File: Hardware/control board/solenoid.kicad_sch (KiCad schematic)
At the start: 7 parts, among them J11 Screw_Terminal_01x02, Q3 NMOS

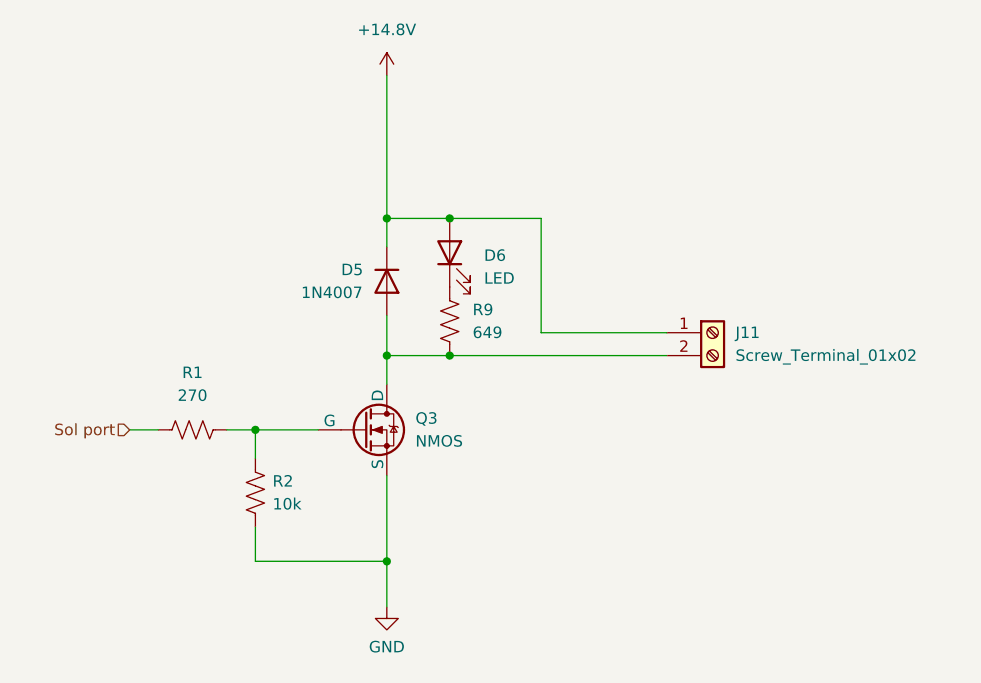
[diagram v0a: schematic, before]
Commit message: schematic formatted
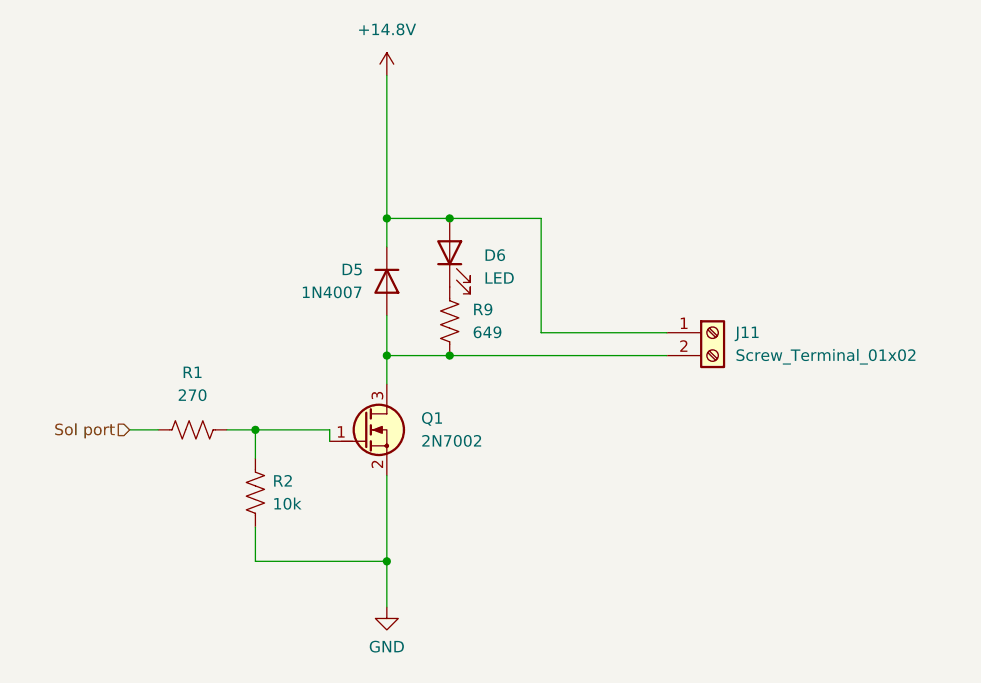
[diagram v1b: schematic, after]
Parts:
- removed Q3: NMOS, symbol Simulation_SPICE:NMOS
- added Q1: 2N7002, Package_TO_SOT_SMD_AKL:SOT-23, symbol PCM_Transistor_MOSFET_AKL:2N7002
- D6: footprint (none) -> LED_THT:LED_D3.0mm
- J11: footprint (none) -> TerminalBlock_Phoenix:TerminalBlock_Phoenix_MPT-0,5-2-2.54_1x02_P2.54mm_Horizontal
- R1, R2, R9: footprint (none) -> Resistor_SMD:R_0805_2012Metric
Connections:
- net GND: now also Q1.2 (S)
- net at D5.2 (A), J11.2 (Pin_2), R9.2: now also Q1.3 (D)
- net at R1.2, R2.1: now also Q1.1 (G)
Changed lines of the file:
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@@
     (stroke (width 0) (type default))
   )
-  (wire (pts (xy 107.95 99.06) (xy 114.935 99.06))
+  (wire (pts (xy 107.95 99.06) (xy 116.205 99.06))
     (stroke (width 0) (type default))
   )
@@
   )
   (wire (pts (xy 122.555 86.36) (xy 122.555 90.805))
+    (stroke (width 0) (type default))
+  )
+  (wire (pts (xy 116.205 99.06) (xy 116.205 100.33))
     (stroke (width 0) (type default))
   )
@@
     (effects (font (size 1.27 1.27)) (justify right))
   )
-  (symbol (lib_id "Simulation_SPICE:NMOS") (at 120.015 99.06 0) (unit 1)
-    (in_bom yes) (on_board yes) (dnp no) (fields_autoplaced)
-    (property "Reference" "Q3" (at 125.73 97.79 0)
-      (effects (font (size 1.27 1.27)) (justify left))
-    )
-    (property "Value" "NMOS" (at 125.73 100.33 0)
-      (effects (font (size 1.27 1.27)) (justify left))
-    )
-    (property "Footprint" "" (at 125.095 96.52 0)
-      (effects (font (size 1.27 1.27)) hide)
-    )
-    (property "Datasheet" "https://ngspice.sourceforge.io/docs/ngspice-manual.pdf" (at 120.015 111.76 0)
-      (effects (font (size 1.27 1.27)) hide)
-    )
-    (property "Sim.Device" "NMOS" (at 120.015 116.205 0)
-      (effects (font (size 1.27 1.27)) hide)
-    )
-    (property "Sim.Type" "VDMOS" (at 120.015 118.11 0)
-      (effects (font (size 1.27 1.27)) hide)
-    )
-    (property "Sim.Pins" "1=D 2=G 3=S" (at 120.015 114.3 0)
-      (effects (font (size 1.27 1.27)) hide)
-    )
-    (pin "1")
-    (pin "2")
-    (pin "3")
-    (instances
-      (project "solenoid"
-        (path "/b4ed5960-473e-41d7-9d87-eb439ed22219"
-          (reference "Q3") (unit 1)
-        )
-      )
-      (project "control board"
-        (path "/cf0863a8-7f64-449b-8eb4-3c06c871fb37"
-          (reference "Q3") (unit 1)
-        )
-        (path "/cf0863a8-7f64-449b-8eb4-3c06c871fb37/9fd0b45f-6f46-40af-ae0d-29c33b45e498"
-          (reference "Q1") (unit 1)
-        )
-        (path "/cf0863a8-7f64-449b-8eb4-3c06c871fb37/6163a064-c95f-47b6-9c17-0e18c391c233"
-          (reference "Q2") (unit 1)
-        )
-        (path "/cf0863a8-7f64-449b-8eb4-3c06c871fb37/f39ce93b-3626-4dde-a021-b00a2c8134c7"
-          (reference "Q3") (unit 1)
-        )
-      )
-    )
-  )
   (symbol (lib_id "Device:LED") (at 129.54 79.375 90) (unit 1)
     (in_bom yes) (on_board yes) (dnp no) (fields_autoplaced)
@@
       (effects (font (size 1.27 1.27)) (justify right))
     )
-    (property "Footprint" "" (at 129.54 79.375 0)
+    (property "Footprint" "LED_THT:LED_D3.0mm" (at 129.54 79.375 0)
       (effects (font (size 1.27 1.27)) hide)
     )
@@
         )
         (path "/cf0863a8-7f64-449b-8eb4-3c06c871fb37/9fd0b45f-6f46-40af-ae0d-29c33b45e498"
-          (reference "Green") (unit 1)
+          (reference "Green1") (unit 1)
         )
         (path "/cf0863a8-7f64-449b-8eb4-3c06c871fb37/6163a064-c95f-47b6-9c17-0e18c391c233"
@@
       (effects (font (size 1.27 1.27)) (justify left))
     )
-    (property "Footprint" "" (at 158.75 88.265 0)
+    (property "Footprint" "TerminalBlock_Phoenix:TerminalBlock_Phoenix_MPT-0,5-2-2.54_1x02_P2.54mm_Horizontal" (at 158.75 88.265 0)
       (effects (font (size 1.27 1.27)) hide)
     )
@@
       (effects (font (size 1.27 1.27)))
     )
-    (property "Footprint" "" (at 101.219 98.044 90)
+    (property "Footprint" "Resistor_SMD:R_0805_2012Metric" (at 101.219 98.044 90)
       (effects (font (size 1.27 1.27)) hide)
     )
@@
       (effects (font (size 1.27 1.27)) (justify left))
     )
-    (property "Footprint" "" (at 108.966 106.299 90)
+    (property "Footprint" "Resistor_SMD:R_0805_2012Metric" (at 108.966 106.299 90)
       (effects (font (size 1.27 1.27)) hide)
     )
@@
       (effects (font (size 1.27 1.27)) (justify left))
     )
-    (property "Footprint" "" (at 130.556 87.249 90)
+    (property "Footprint" "Resistor_SMD:R_0805_2012Metric" (at 130.556 87.249 90)
       (effects (font (size 1.27 1.27)) hide)
     )
@@
         )
       )
+    )
+  )
+  (symbol (lib_id "PCM_Transistor_MOSFET_AKL:2N7002") (at 120.015 99.06 0) (unit 1)
+    (in_bom yes) (on_board yes) (dnp no) (fields_autoplaced)
+    (property "Reference" "Q1" (at 126.365 97.79 0)
+      (effects (font (size 1.27 1.27)) (justify left))
+    )
+    (property "Value" "2N7002" (at 126.365 100.33 0)
+      (effects (font (size 1.27 1.27)) (justify left))
+    )
+    (property "Footprint" "Package_TO_SOT_SMD_AKL:SOT-23" (at 125.095 96.52 0)
+      (effects (font (size 1.27 1.27)) hide)
+    )
+    (property "Datasheet" "https://www.tme.eu/Document/7df5cae36abdfcedddb681f5be886f05/2N7000.pdf" (at 120.015 99.06 0)
+      (effects (font (size 1.27 1.27)) hide)
+    )
+    (pin "1")
+    (pin "2")
+    (pin "3")
+    (instances
+      (project "control board"
+        (path "/cf0863a8-7f64-449b-8eb4-3c06c871fb37/9fd0b45f-6f46-40af-ae0d-29c33b45e498"
+          (reference "Q1") (unit 1)
+        )
+        (path "/cf0863a8-7f64-449b-8eb4-3c06c871fb37/6163a064-c95f-47b6-9c17-0e18c391c233"
+          (reference "Q2") (unit 1)
+        )
+        (path "/cf0863a8-7f64-449b-8eb4-3c06c871fb37/f39ce93b-3626-4dde-a021-b00a2c8134c7"
+          (reference "Q3") (unit 1)
+        )
+      )

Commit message: Revert "Merge branch 'hardware' of https://github.com/bruin-underwater-robotics/2023-2024 into hardware"
This reverts commit f5050c74fbd2d727488e15b71bfb24c9149407df, reversing
changes made to d4ffa11f2369dfdbeb25d57bd1642de1ab50c466.
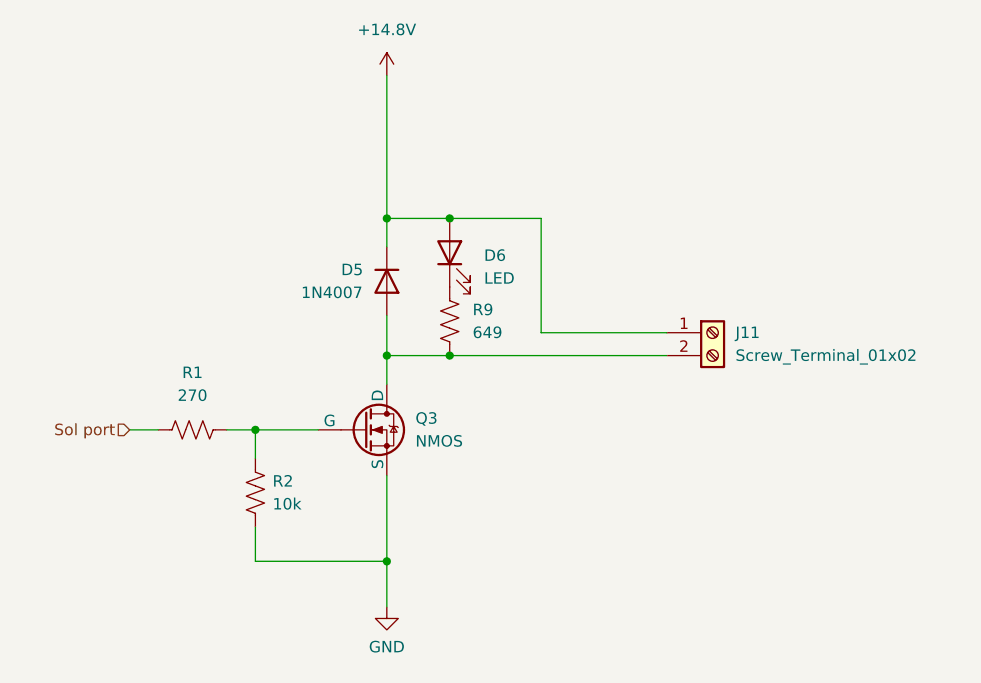
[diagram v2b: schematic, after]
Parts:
- removed Q1: 2N7002, Package_TO_SOT_SMD_AKL:SOT-23, symbol PCM_Transistor_MOSFET_AKL:2N7002
- added Q3: NMOS, symbol Simulation_SPICE:NMOS
- D6: footprint LED_THT:LED_D3.0mm -> (none)
- J11: footprint TerminalBlock_Phoenix:TerminalBlock_Phoenix_MPT-0,5-2-2.54_1x02_P2.54mm_Horizontal -> (none)
- R1, R2, R9: footprint Resistor_SMD:R_0805_2012Metric -> (none)
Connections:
- net GND: now also Q3.3 (S)
- net at D5.2 (A), J11.2 (Pin_2), R9.2: now also Q3.1 (D)
- net at R1.2, R2.1: now also Q3.2 (G)
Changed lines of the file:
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@@
     (stroke (width 0) (type default))
   )
-  (wire (pts (xy 107.95 99.06) (xy 116.205 99.06))
+  (wire (pts (xy 107.95 99.06) (xy 114.935 99.06))
     (stroke (width 0) (type default))
   )
@@
   )
   (wire (pts (xy 122.555 86.36) (xy 122.555 90.805))
-    (stroke (width 0) (type default))
-  )
-  (wire (pts (xy 116.205 99.06) (xy 116.205 100.33))
     (stroke (width 0) (type default))
   )
@@
     (effects (font (size 1.27 1.27)) (justify right))
   )
+  (symbol (lib_id "Simulation_SPICE:NMOS") (at 120.015 99.06 0) (unit 1)
+    (in_bom yes) (on_board yes) (dnp no) (fields_autoplaced)
+    (property "Reference" "Q3" (at 125.73 97.79 0)
+      (effects (font (size 1.27 1.27)) (justify left))
+    )
+    (property "Value" "NMOS" (at 125.73 100.33 0)
+      (effects (font (size 1.27 1.27)) (justify left))
+    )
+    (property "Footprint" "" (at 125.095 96.52 0)
+      (effects (font (size 1.27 1.27)) hide)
+    )
+    (property "Datasheet" "https://ngspice.sourceforge.io/docs/ngspice-manual.pdf" (at 120.015 111.76 0)
+      (effects (font (size 1.27 1.27)) hide)
+    )
+    (property "Sim.Device" "NMOS" (at 120.015 116.205 0)
+      (effects (font (size 1.27 1.27)) hide)
+    )
+    (property "Sim.Type" "VDMOS" (at 120.015 118.11 0)
+      (effects (font (size 1.27 1.27)) hide)
+    )
+    (property "Sim.Pins" "1=D 2=G 3=S" (at 120.015 114.3 0)
+      (effects (font (size 1.27 1.27)) hide)
+    )
+    (pin "1")
+    (pin "2")
+    (pin "3")
+    (instances
+      (project "solenoid"
+        (path "/b4ed5960-473e-41d7-9d87-eb439ed22219"
+          (reference "Q3") (unit 1)
+        )
+      )
+      (project "control board"
+        (path "/cf0863a8-7f64-449b-8eb4-3c06c871fb37"
+          (reference "Q3") (unit 1)
+        )
+        (path "/cf0863a8-7f64-449b-8eb4-3c06c871fb37/9fd0b45f-6f46-40af-ae0d-29c33b45e498"
+          (reference "Q1") (unit 1)
+        )
+        (path "/cf0863a8-7f64-449b-8eb4-3c06c871fb37/6163a064-c95f-47b6-9c17-0e18c391c233"
+          (reference "Q2") (unit 1)
+        )
+        (path "/cf0863a8-7f64-449b-8eb4-3c06c871fb37/f39ce93b-3626-4dde-a021-b00a2c8134c7"
+          (reference "Q3") (unit 1)
+        )
+      )
+    )
+  )
   (symbol (lib_id "Device:LED") (at 129.54 79.375 90) (unit 1)
     (in_bom yes) (on_board yes) (dnp no) (fields_autoplaced)
@@
       (effects (font (size 1.27 1.27)) (justify right))
     )
-    (property "Footprint" "LED_THT:LED_D3.0mm" (at 129.54 79.375 0)
+    (property "Footprint" "" (at 129.54 79.375 0)
       (effects (font (size 1.27 1.27)) hide)
     )
@@
         )
         (path "/cf0863a8-7f64-449b-8eb4-3c06c871fb37/9fd0b45f-6f46-40af-ae0d-29c33b45e498"
-          (reference "Green1") (unit 1)
+          (reference "Green") (unit 1)
         )
         (path "/cf0863a8-7f64-449b-8eb4-3c06c871fb37/6163a064-c95f-47b6-9c17-0e18c391c233"
@@
       (effects (font (size 1.27 1.27)) (justify left))
     )
-    (property "Footprint" "TerminalBlock_Phoenix:TerminalBlock_Phoenix_MPT-0,5-2-2.54_1x02_P2.54mm_Horizontal" (at 158.75 88.265 0)
+    (property "Footprint" "" (at 158.75 88.265 0)
       (effects (font (size 1.27 1.27)) hide)
     )
@@
       (effects (font (size 1.27 1.27)))
     )
-    (property "Footprint" "Resistor_SMD:R_0805_2012Metric" (at 101.219 98.044 90)
+    (property "Footprint" "" (at 101.219 98.044 90)
       (effects (font (size 1.27 1.27)) hide)
     )
@@
       (effects (font (size 1.27 1.27)) (justify left))
     )
-    (property "Footprint" "Resistor_SMD:R_0805_2012Metric" (at 108.966 106.299 90)
+    (property "Footprint" "" (at 108.966 106.299 90)
       (effects (font (size 1.27 1.27)) hide)
     )
@@
       (effects (font (size 1.27 1.27)) (justify left))
     )
-    (property "Footprint" "Resistor_SMD:R_0805_2012Metric" (at 130.556 87.249 90)
+    (property "Footprint" "" (at 130.556 87.249 90)
       (effects (font (size 1.27 1.27)) hide)
     )
@@
         )
       )
-    )
-  )
-  (symbol (lib_id "PCM_Transistor_MOSFET_AKL:2N7002") (at 120.015 99.06 0) (unit 1)
-    (in_bom yes) (on_board yes) (dnp no) (fields_autoplaced)
-    (property "Reference" "Q1" (at 126.365 97.79 0)
-      (effects (font (size 1.27 1.27)) (justify left))
-    )
-    (property "Value" "2N7002" (at 126.365 100.33 0)
-      (effects (font (size 1.27 1.27)) (justify left))
-    )
-    (property "Footprint" "Package_TO_SOT_SMD_AKL:SOT-23" (at 125.095 96.52 0)
-      (effects (font (size 1.27 1.27)) hide)
-    )
-    (property "Datasheet" "https://www.tme.eu/Document/7df5cae36abdfcedddb681f5be886f05/2N7000.pdf" (at 120.015 99.06 0)
-      (effects (font (size 1.27 1.27)) hide)
-    )
-    (pin "1")
-    (pin "2")
-    (pin "3")
-    (instances
-      (project "control board"
-        (path "/cf0863a8-7f64-449b-8eb4-3c06c871fb37/9fd0b45f-6f46-40af-ae0d-29c33b45e498"
-          (reference "Q1") (unit 1)
-        )
-        (path "/cf0863a8-7f64-449b-8eb4-3c06c871fb37/6163a064-c95f-47b6-9c17-0e18c391c233"
-          (reference "Q2") (unit 1)
-        )
-        (path "/cf0863a8-7f64-449b-8eb4-3c06c871fb37/f39ce93b-3626-4dde-a021-b00a2c8134c7"
-          (reference "Q3") (unit 1)
-        )
-      )

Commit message: fixing stupid mistakes
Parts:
- D6: footprint (none) -> LED_THT:LED_D3.0mm
- J11: footprint (none) -> Library:TE_282836-2
- Q3: footprint (none) -> PCM_Package_TO_SOT_SMD_AKL:TSOT-23_BigPads
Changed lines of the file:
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@@
       (effects (font (size 1.27 1.27)) (justify left))
     )
-    (property "Footprint" "" (at 125.095 96.52 0)
+    (property "Footprint" "PCM_Package_TO_SOT_SMD_AKL:TSOT-23_BigPads" (at 125.095 96.52 0)
       (effects (font (size 1.27 1.27)) hide)
     )
@@
       (effects (font (size 1.27 1.27)) (justify right))
     )
-    (property "Footprint" "" (at 129.54 79.375 0)
+    (property "Footprint" "LED_THT:LED_D3.0mm" (at 129.54 79.375 0)
       (effects (font (size 1.27 1.27)) hide)
     )
@@
         )
         (path "/cf0863a8-7f64-449b-8eb4-3c06c871fb37/9fd0b45f-6f46-40af-ae0d-29c33b45e498"
-          (reference "Green") (unit 1)
+          (reference "Green1") (unit 1)
         )
         (path "/cf0863a8-7f64-449b-8eb4-3c06c871fb37/6163a064-c95f-47b6-9c17-0e18c391c233"
@@
       (effects (font (size 1.27 1.27)) (justify left))
     )
-    (property "Footprint" "" (at 158.75 88.265 0)
+    (property "Footprint" "Library:TE_282836-2" (at 158.75 88.265 0)
       (effects (font (size 1.27 1.27)) hide)
     )

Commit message: footprint work
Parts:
- R1, R2, R9: footprint (none) -> Resistor_SMD:R_0805_2012Metric
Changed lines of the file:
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@@
       (effects (font (size 1.27 1.27)))
     )
-    (property "Footprint" "" (at 101.219 98.044 90)
+    (property "Footprint" "Resistor_SMD:R_0805_2012Metric" (at 101.219 98.044 90)
       (effects (font (size 1.27 1.27)) hide)
     )
@@
       (effects (font (size 1.27 1.27)) (justify left))
     )
-    (property "Footprint" "" (at 108.966 106.299 90)
+    (property "Footprint" "Resistor_SMD:R_0805_2012Metric" (at 108.966 106.299 90)
       (effects (font (size 1.27 1.27)) hide)
     )
@@
       (effects (font (size 1.27 1.27)) (justify left))
     )
-    (property "Footprint" "" (at 130.556 87.249 90)
+    (property "Footprint" "Resistor_SMD:R_0805_2012Metric" (at 130.556 87.249 90)
       (effects (font (size 1.27 1.27)) hide)
     )

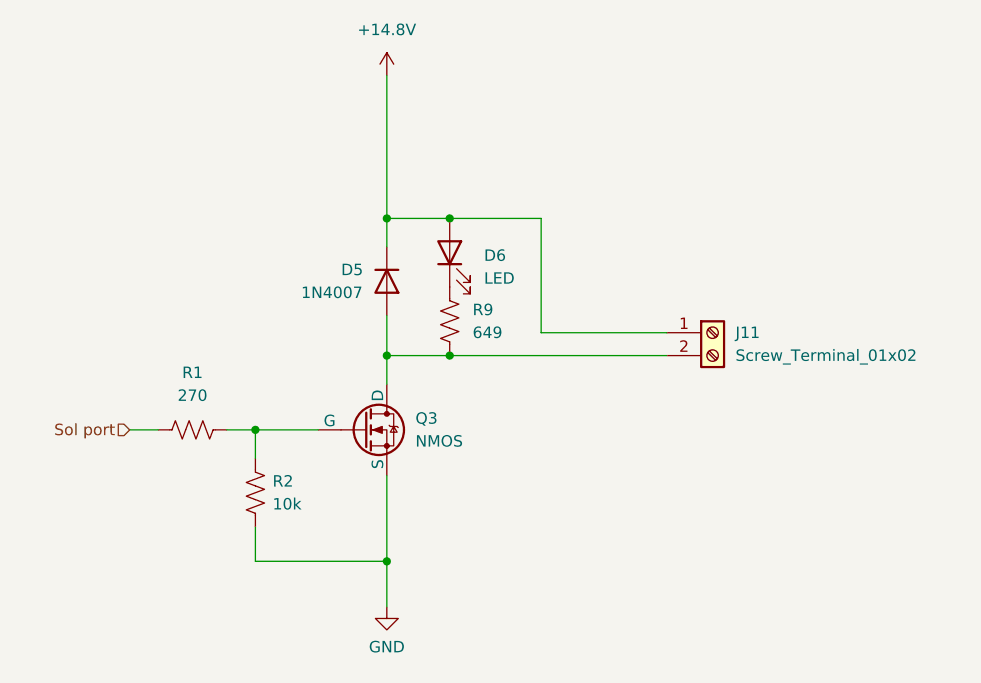
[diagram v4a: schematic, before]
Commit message: control board clean up
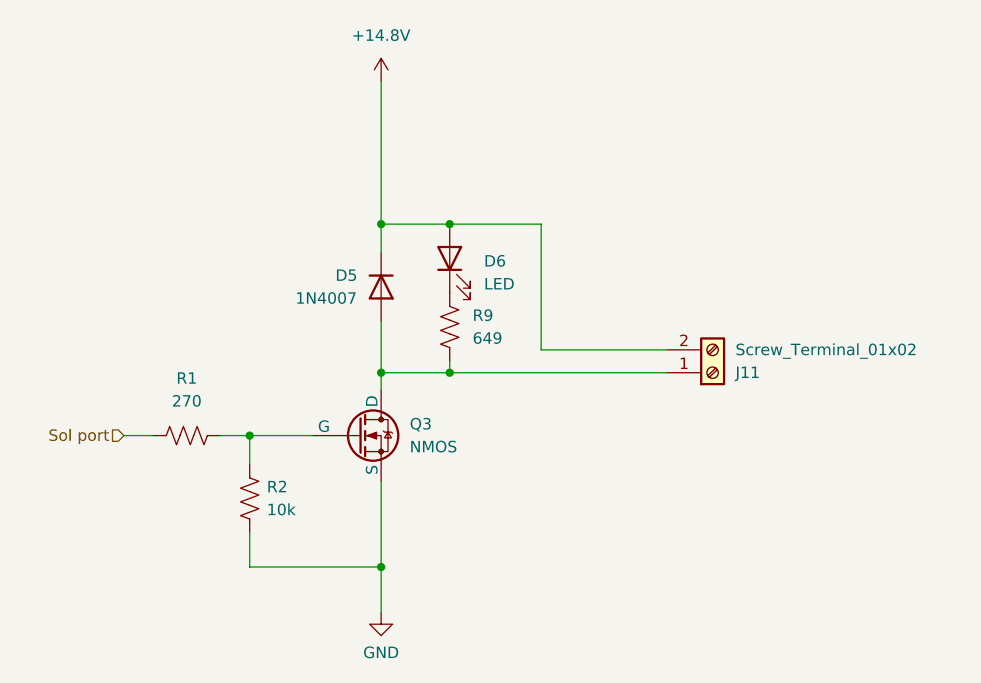
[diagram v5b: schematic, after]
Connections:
- net +14.8V: now also J11.2 (Pin_2); no longer J11.1 (Pin_1)
- net at D5.2 (A), Q3.1 (D), R9.2: now also J11.1 (Pin_1); no longer J11.2 (Pin_2)
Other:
- moved on the sheet: D5, D6, J11, Q3, R1, R2, R9
